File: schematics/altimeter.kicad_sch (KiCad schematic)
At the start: 6 parts, among them U4 TXB0106, U5 MS5611-01BA, U6 ICM-20948

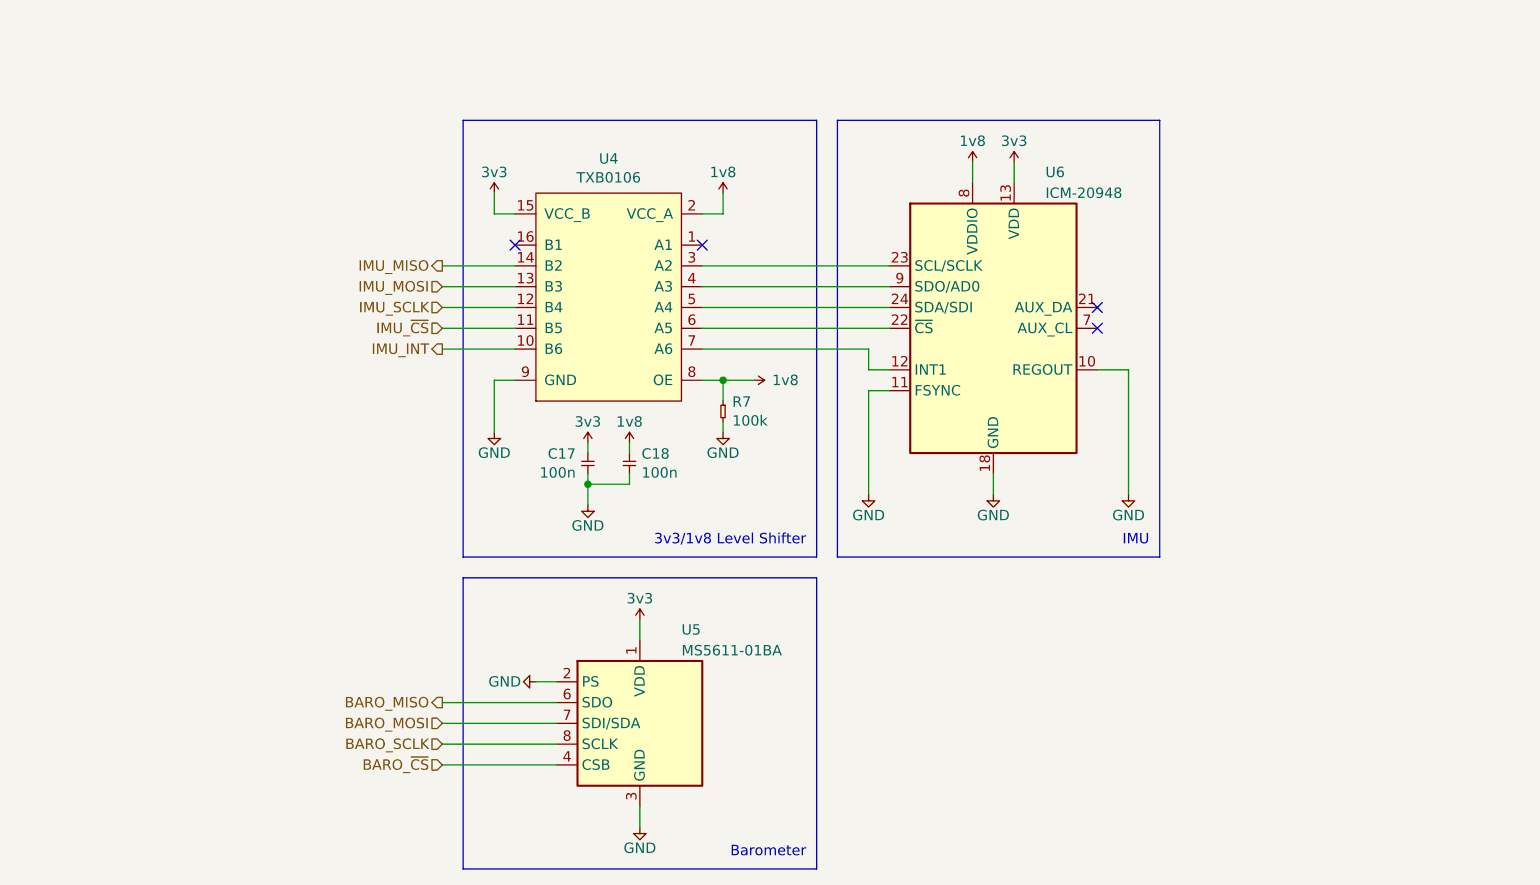
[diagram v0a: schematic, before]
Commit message: Complete revision 1 schematic
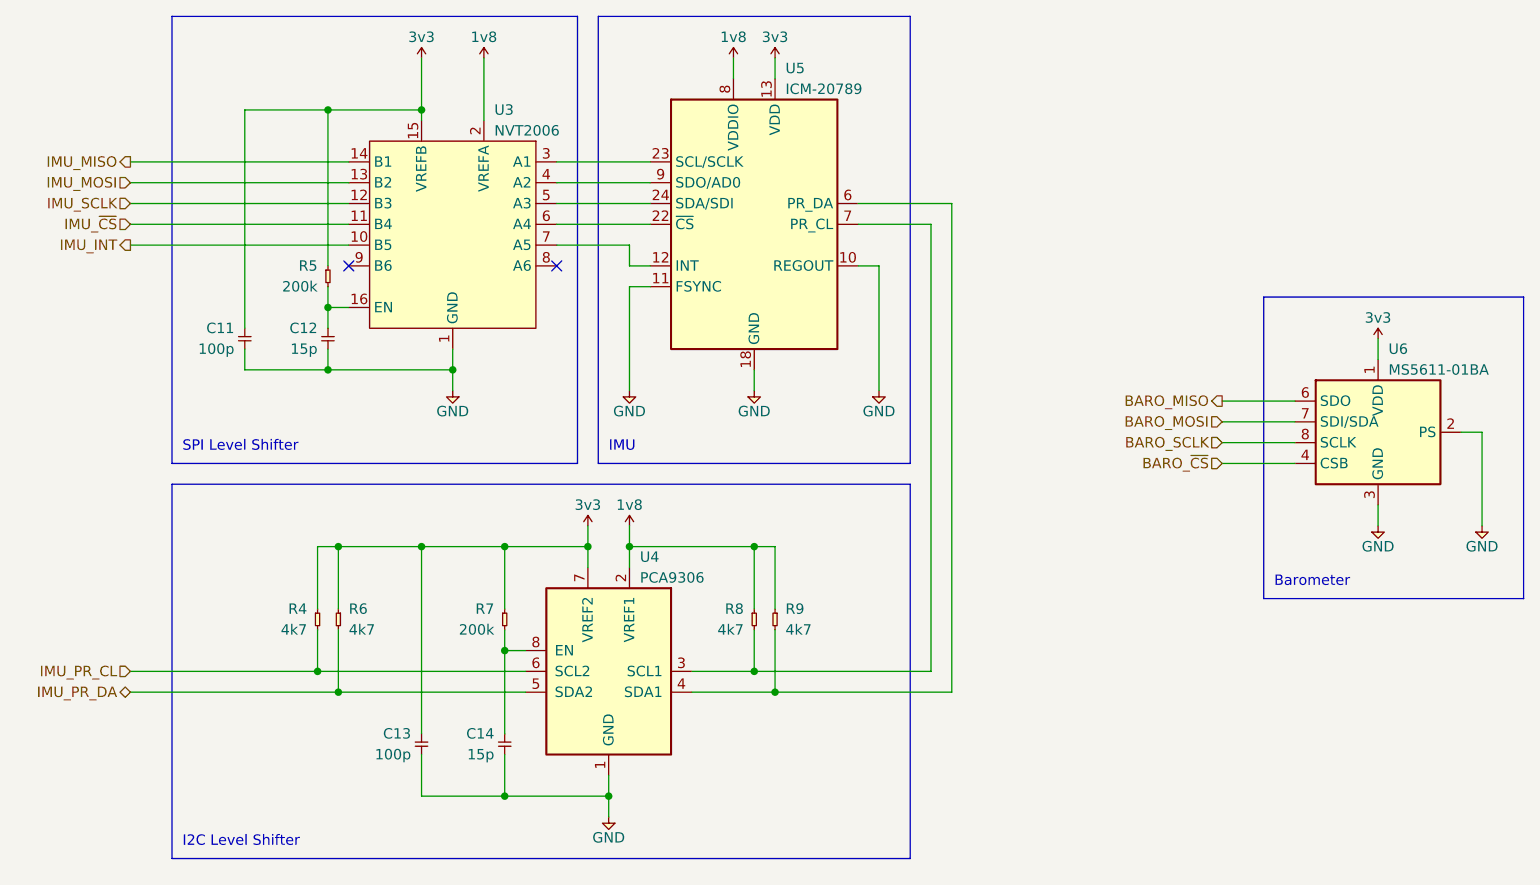
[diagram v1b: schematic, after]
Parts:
- removed C17, C18: 100n, Strix:C_0402, symbol Strix:C
- removed U4: TXB0106, symbol Strix:TXB0106
- removed U5: MS5611-01BA, Strix:MS5611-01BA, symbol Strix:MS5611-01BA
- removed U6: ICM-20948, Strix:ICM-20948, symbol Strix:ICM-20948
- added C11, C13: 100p, symbol Strix:C
- added C12, C14: 15p, symbol Strix:C
- added R4, R6, R8, R9: 4k7, symbol Strix:R
- added R5: 200k, symbol Strix:R
- added U3: NVT2006, symbol Strix:NVT2006
- added U4: PCA9306, symbol Strix:PCA9306
- added U5: ICM-20789, Strix:ICM-20789, symbol Strix:ICM-20789
- added U6: MS5611-01BA, Strix:MS5611-01BA, symbol Strix:MS5611-01BA
- R7: value 100k -> 200k; footprint Strix:R_0402 -> (none)
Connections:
- net 1v8: now also R8.1, R9.1, U3.2 (VREFA), U4.2 (VREF1), U5.8 (VDDIO); no longer R7.1
- net 3v3: now also R7.1, C11.2, C13.2, R4.1, R5.1, R6.1, U3.15 (VREFB), U4.7 (VREF2), U5.13 (VDD), U6.1 (VDD)
- net BARO_MISO: now also U6.6 (SDO)
- net BARO_MOSI: now also U6.7 (SDI/SDA)
- net BARO_SCLK: now also U6.8 (SCLK)
- net BARO_~{CS}: now also U6.4 (CSB), U6.5 (CSB)
- net GND: now also C11.1, C12.1, C13.1, C14.1, U3.1 (GND), U4.1 (GND), U5.10 (REGOUT), U5.11 (FSYNC), U5.18 (GND), U5.20 (NC), U6.2 (PS), U6.3 (GND); no longer R7.2
- net IMU_INT: now also U3.10 (B5)
- net IMU_MISO: now also U3.14 (B1)
- net IMU_MOSI: now also U3.13 (B2)
- net IMU_SCLK: now also U3.12 (B3)
- net IMU_~{CS}: now also U3.11 (B4)
- new net: C12.2, R5.2, U3.16 (EN)
- new net: U3.3 (A1), U5.23 (SCL/SCLK)
- new net: U3.4 (A2), U5.9 (SDO/AD0)
- new net: U3.5 (A3), U5.24 (SDA/SDI)
- new net: U3.6 (A4), U5.22 (~{CS})
- new net: U3.7 (A5), U5.12 (INT)
- new net: C14.2, R7.2, U4.8 (EN)
- new net: R9.2, U4.4 (SDA1), U5.6 (PR_DA)
- new net: R8.2, U4.3 (SCL1), U5.7 (PR_CL)
- new net IMU_PR_CL: R4.2, U4.6 (SCL2)
- new net IMU_PR_DA: R6.2, U4.5 (SDA2)
- no-connect marks 4 -> 2
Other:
- note added: "I2C Level Shifter"
- note added: "SPI Level Shifter"
- note removed: "3v3/1v8 Level Shifter"
